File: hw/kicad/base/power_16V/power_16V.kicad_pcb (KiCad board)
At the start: 2 copper layers, 40 x 40 mm, 34 parts, among them J1 USB_B_Micro, J3 TOP, J4 BUTTOM, U1 LM2596S-5, U2 LM1117MP-3.3, U3 CP2104

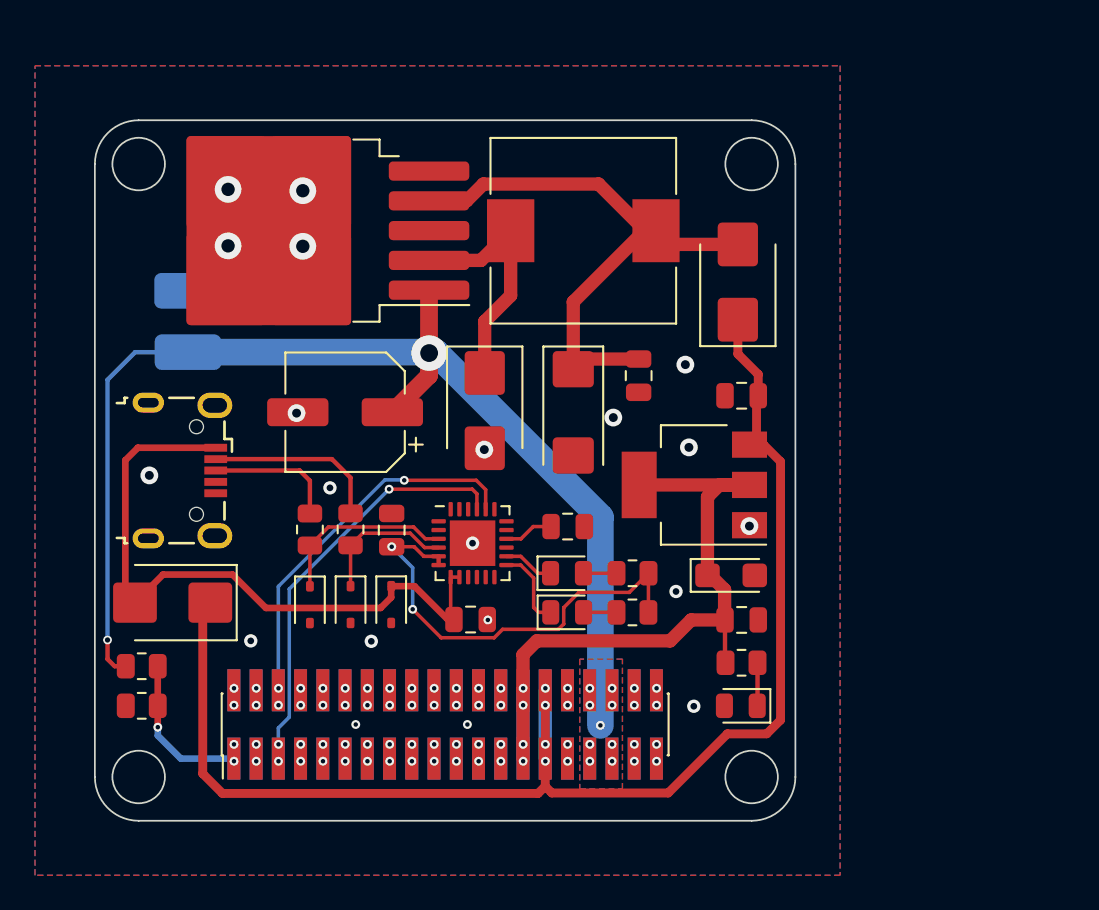
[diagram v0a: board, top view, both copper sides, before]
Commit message: Merge from normal
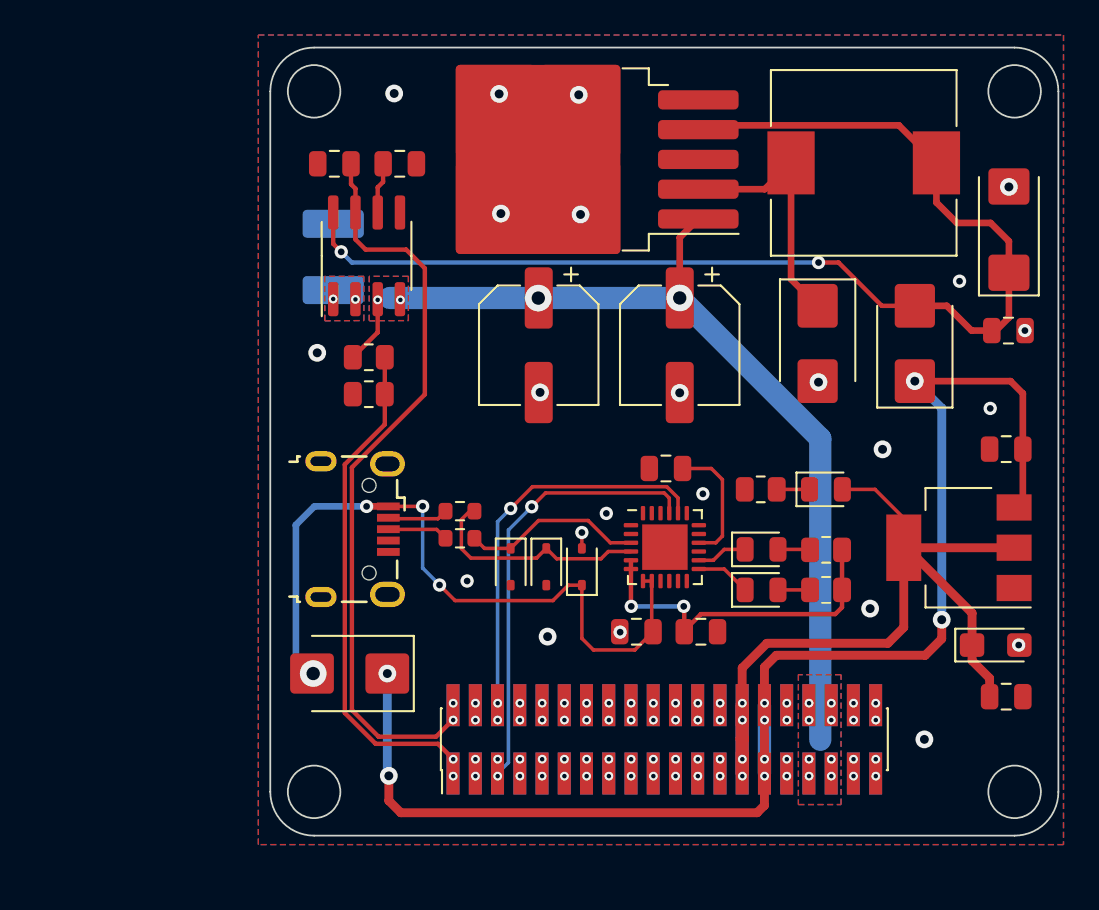
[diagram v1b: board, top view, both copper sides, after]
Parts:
- removed the ? at (46.0, 46.6)
- removed the ? at (46.0, 50.1)
- added ?: , , B.Cu at (54.3, 46.6)
- added ?: , , B.Cu at (54.3, 42.8)
- added C10: 220uF, Capacitor_SMD:CP_Elec_6.3x7.7, F.Cu at (66.0, 49.7)
- added C11: 0.1uF, Capacitor_SMD:C_0805_2012Metric, F.Cu at (58.1, 39.4)
- added C12: 0.1uF, Capacitor_SMD:C_0805_2012Metric, F.Cu at (54.4, 39.4)
- added U4: ACS712xLCTR-05B, Package_SO:SOIC-8_3.9x4.9mm_P1.27mm, F.Cu at (56.2, 44.6)
- C1: value 100uF -> 220uF
- R1, R2: footprint Resistor_SMD:R_0805_2012Metric -> Resistor_SMD:R_0603_1608Metric
- R4, R5: value 22 -> 100
- moved C7 27.0 mm to (92.9, 43.1), turned to 90 degrees
- moved R7 22.0 mm to (56.3, 52.5)
- moved R6 21.9 mm to (56.3, 50.4)
- moved C8 21.3 mm to (92.9, 48.9), turned to 0 degrees
- moved C1 19.5 mm to (74.1, 49.7), turned to -90 degrees
- moved D3 19.4 mm to (82.0, 49.6)
- moved C9 18.6 mm to (75.3, 66.1), turned to 180 degrees
- moved L1 16.5 mm to (84.6, 39.3)
- moved U1 15.9 mm to (67.5, 39.1)
- moved C6 15.7 mm to (92.7, 69.8)
- moved C3 15.6 mm to (92.1, 66.8)
- moved U2 15.5 mm to (90.0, 61.3)
- moved C2 15.4 mm to (92.7, 55.6)
- moved D7 13.3 mm to (82.4, 57.9), turned to 0 degrees
- moved J3 12.5 mm to (73.2, 72.2)
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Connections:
- net Net-(D6-A) renamed /DCDC_+5V
- D7 pad 2: GND -> +3.3V
- J3 pad 10: /I2C_CLK -> /UART3_Tx
- J3 pad 11: /SPI_CS -> /I2C_SDA
- J3 pad 12: /SPI_CLK -> /I2C_CLK
- J3 pad 13: /SPI_MOSI -> /SPI_CS
- J3 pad 14: /SPI_MISO -> /SPI_CLK
- J3 pad 15: /GPIO_1 -> /SPI_MOSI
- J3 pad 16: /GPIO_2 -> /SPI_MISO
- J3 pad 17: /GPIO_3 -> /GPIO_1
- J3 pad 18: /GPIO_4 -> /GPIO_2
- J3 pad 19: /GPIO_5 -> /GPIO_3
- J3 pad 20: /GPIO_6 -> /GPIO_4
- J3 pad 21: /GPIO_7 -> /GPIO_5
- J3 pad 22: /GPIO_8 -> /GPIO_6
- J3 pad 23: /GPIO_9 -> /GPIO_7
- J3 pad 24: /GPIO_10 -> /GPIO_8
- J3 pad 25: /GPIO_11 -> /GPIO_9
- J3 pad 26: /GPIO_12 -> /GPIO_10
- J3 pad 9: /I2C_SDA -> /UART3_Rx
- J4 pad 10: /I2C_SDA -> /UART3_Rx
- J4 pad 11: /SPI_CLK -> /I2C_CLK
- J4 pad 12: /SPI_CS -> /I2C_SDA
- J4 pad 13: /SPI_MISO -> /SPI_CLK
- J4 pad 14: /SPI_MOSI -> /SPI_CS
- J4 pad 15: /GPIO_2 -> /SPI_MISO
- J4 pad 16: /GPIO_1 -> /SPI_MOSI
- J4 pad 17: /GPIO_4 -> /GPIO_2
- J4 pad 18: /GPIO_3 -> /GPIO_1
- J4 pad 19: /GPIO_6 -> /GPIO_4
- J4 pad 20: /GPIO_5 -> /GPIO_3
- J4 pad 21: /GPIO_8 -> /GPIO_6
- J4 pad 22: /GPIO_7 -> /GPIO_5
- J4 pad 23: /GPIO_10 -> /GPIO_8
- J4 pad 24: /GPIO_9 -> /GPIO_7
- J4 pad 25: /GPIO_12 -> /GPIO_10
- J4 pad 26: /GPIO_11 -> /GPIO_9
- J4 pad 9: /I2C_CLK -> /UART3_Tx
- R3 pad 1: +3.3V -> GND
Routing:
- net /ADC_2: track 0.00 -> 43.7 mm
- net /DCDC_+5V: track 33.7 -> 69.0 mm, vias 0 -> 2
- net /ADC_1: track 8.85 -> 29.4 mm, vias 3 -> 2
- net +BATT: track 69.6 -> 54.2 mm, vias 11 -> 12
- net +3.3V: track 41.2 -> 49.4 mm
- net Net-(J1-D-): track 10.2 -> 3.43 mm
- net /VIO: track 25.9 -> 20.0 mm
- net Net-(D4-K): track 7.99 -> 13.2 mm
- net Net-(U3-VPP): track 2.83 -> 7.27 mm
- net Net-(J1-D+): track 7.49 -> 3.50 mm
- net Net-(D1-A): track 38.2 -> 41.6 mm, vias 0 -> 4
- net Net-(U4-FILTER): track 0.00 -> 2.91 mm
- net +5V: track 79.6 -> 82.5 mm, vias 4 -> 8
- net Net-(D8-K): track 4.63 -> 3.14 mm
- net /UART1_Rx: track 24.0 -> 25.2 mm
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- added copper zone on B.Cu, net /+BATT_IN
- added copper zone on F.Cu, net /+BATT_IN
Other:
- board size 40 x 40 mm -> 45 x 45 mm
- board text added: "Pindar v1.2 (Base) power16v v1.2"
- board text removed: "Pindar v1.3 Type BASE power16v v1.2"
